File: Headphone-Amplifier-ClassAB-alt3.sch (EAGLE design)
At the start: 17 parts, among them T1 2N3904, T2 2N3904, T3 2N3906

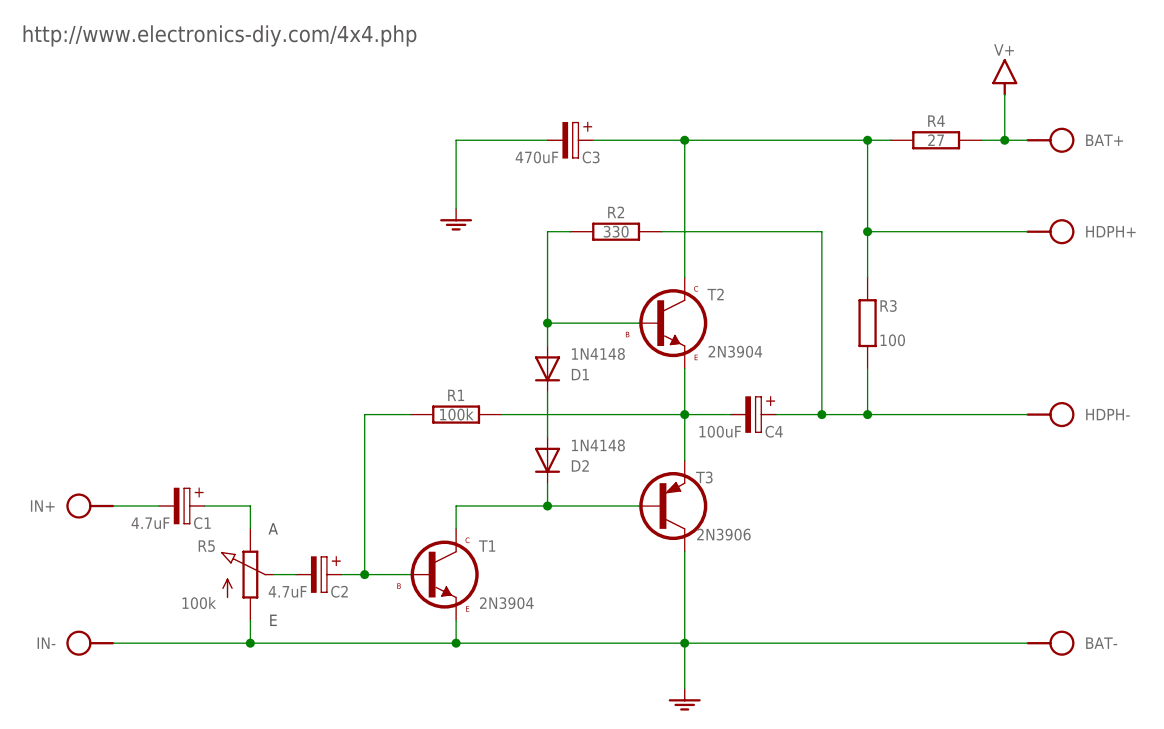
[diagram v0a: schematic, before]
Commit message: ...
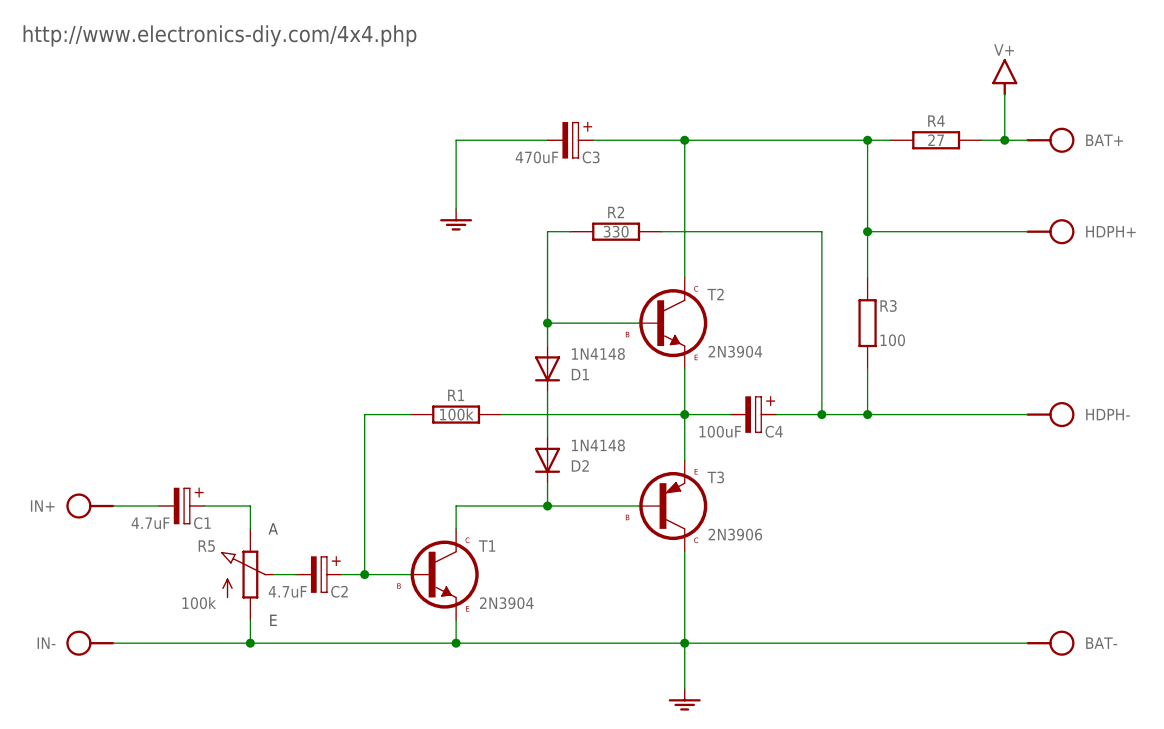
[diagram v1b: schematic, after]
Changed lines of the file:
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@@
     <grid distance="0.1" unitdist="inch" unit="inch" style="lines" multiple="1" display="yes" altdistance="2" altunitdist="inch" altunit="inch" />
     <layers>
-      <layer number="1" name="Top" color="4" fill="1" visible="yes" active="no" />
-      <layer number="2" name="Route2" color="1" fill="3" visible="yes" active="no" />
-      <layer number="3" name="Route3" color="4" fill="3" visible="yes" active="no" />
-      <layer number="4" name="Route4" color="1" fill="4" visible="yes" active="no" />
-      <layer number="5" name="Route5" color="4" fill="4" visible="yes" active="no" />
-      <layer number="6" name="Route6" color="1" fill="8" visible="yes" active="no" />
-      <layer number="7" name="Route7" color="4" fill="8" visible="yes" active="no" />
-      <layer number="8" name="Route8" color="1" fill="2" visible="yes" active="no" />
-      <layer number="9" name="Route9" color="4" fill="2" visible="yes" active="no" />
-      <layer number="10" name="Route10" color="1" fill="7" visible="yes" active="no" />
-      <layer number="11" name="Route11" color="4" fill="7" visible="yes" active="no" />
-      <layer number="12" name="Route12" color="1" fill="5" visible="yes" active="no" />
-      <layer number="13" name="Route13" color="4" fill="5" visible="yes" active="no" />
-      <layer number="14" name="Route14" color="1" fill="6" visible="yes" active="no" />
-      <layer number="15" name="Route15" color="4" fill="6" visible="yes" active="no" />
-      <layer number="16" name="Bottom" color="1" fill="1" visible="yes" active="no" />
-      <layer number="17" name="Pads" color="2" fill="1" visible="yes" active="no" />
-      <layer number="18" name="Vias" color="2" fill="1" visible="yes" active="no" />
-      <layer number="19" name="Unrouted" color="6" fill="1" visible="yes" active="no" />
-      <layer number="20" name="Dimension" color="24" fill="1" visible="yes" active="no" />
-      <layer number="21" name="tPlace" color="16" fill="1" visible="yes" active="no" />
-      <layer number="22" name="bPlace" color="14" fill="1" visible="yes" active="no" />
-      <layer number="23" name="tOrigins" color="15" fill="1" visible="yes" active="no" />
-      <layer number="24" name="bOrigins" color="15" fill="1" visible="yes" active="no" />
-      <layer number="25" name="tNames" color="7" fill="1" visible="yes" active="no" />
-      <layer number="26" name="bNames" color="7" fill="1" visible="yes" active="no" />
-      <layer number="27" name="tValues" color="7" fill="1" visible="yes" active="no" />
-      <layer number="28" name="bValues" color="7" fill="1" visible="yes" active="no" />
+      <layer number="1" name="Top" color="4" fill="1" visible="no" active="no" />
+      <layer number="2" name="Route2" color="1" fill="3" visible="no" active="no" />
+      <layer number="3" name="Route3" color="4" fill="3" visible="no" active="no" />
+      <layer number="4" name="Route4" color="1" fill="4" visible="no" active="no" />
+      <layer number="5" name="Route5" color="4" fill="4" visible="no" active="no" />
+      <layer number="6" name="Route6" color="1" fill="8" visible="no" active="no" />
+      <layer number="7" name="Route7" color="4" fill="8" visible="no" active="no" />
+      <layer number="8" name="Route8" color="1" fill="2" visible="no" active="no" />
+      <layer number="9" name="Route9" color="4" fill="2" visible="no" active="no" />
+      <layer number="10" name="Route10" color="1" fill="7" visible="no" active="no" />
+      <layer number="11" name="Route11" color="4" fill="7" visible="no" active="no" />
+      <layer number="12" name="Route12" color="1" fill="5" visible="no" active="no" />
+      <layer number="13" name="Route13" color="4" fill="5" visible="no" active="no" />
+      <layer number="14" name="Route14" color="1" fill="6" visible="no" active="no" />
+      <layer number="15" name="Route15" color="4" fill="6" visible="no" active="no" />
+      <layer number="16" name="Bottom" color="1" fill="1" visible="no" active="no" />
+      <layer number="17" name="Pads" color="2" fill="1" visible="no" active="no" />
+      <layer number="18" name="Vias" color="2" fill="1" visible="no" active="no" />
+      <layer number="19" name="Unrouted" color="6" fill="1" visible="no" active="no" />
+      <layer number="20" name="Dimension" color="24" fill="1" visible="no" active="no" />
+      <layer number="21" name="tPlace" color="16" fill="1" visible="no" active="no" />
+      <layer number="22" name="bPlace" color="14" fill="1" visible="no" active="no" />
+      <layer number="23" name="tOrigins" color="15" fill="1" visible="no" active="no" />
+      <layer number="24" name="bOrigins" color="15" fill="1" visible="no" active="no" />
+      <layer number="25" name="tNames" color="7" fill="1" visible="no" active="no" />
+      <layer number="26" name="bNames" color="7" fill="1" visible="no" active="no" />
+      <layer number="27" name="tValues" color="7" fill="1" visible="no" active="no" />
+      <layer number="28" name="bValues" color="7" fill="1" visible="no" active="no" />
       <layer number="29" name="tStop" color="7" fill="3" visible="no" active="no" />
       <layer number="30" name="bStop" color="7" fill="6" visible="no" active="no" />
@@
       <layer number="35" name="tGlue" color="7" fill="4" visible="no" active="no" />
       <layer number="36" name="bGlue" color="7" fill="5" visible="no" active="no" />
-      <layer number="37" name="tTest" color="7" fill="1" visible="yes" active="no" />
-      <layer number="38" name="bTest" color="7" fill="1" visible="yes" active="no" />
+      <layer number="37" name="tTest" color="7" fill="1" visible="no" active="no" />
+      <layer number="38" name="bTest" color="7" fill="1" visible="no" active="no" />
       <layer number="39" name="tKeepout" color="4" fill="11" visible="no" active="no" />
       <layer number="40" name="bKeepout" color="1" fill="11" visible="no" active="no" />
@@
       <layer number="44" name="Drills" color="7" fill="1" visible="no" active="no" />
       <layer number="45" name="Holes" color="7" fill="1" visible="no" active="no" />
-      <layer number="46" name="Milling" color="3" fill="1" visible="yes" active="no" />
-      <layer number="47" name="Measures" color="7" fill="1" visible="yes" active="no" />
-      <layer number="48" name="Document" color="7" fill="1" visible="yes" active="no" />
-      <layer number="49" name="Reference" color="7" fill="1" visible="yes" active="no" />
-      <layer number="51" name="tDocu" color="6" fill="1" visible="yes" active="no" />
-      <layer number="52" name="bDocu" color="7" fill="1" visible="yes" active="no" />
+      <layer number="46" name="Milling" color="3" fill="1" visible="no" active="no" />
+      <layer number="47" name="Measures" color="7" fill="1" visible="no" active="no" />
+      <layer number="48" name="Document" color="7" fill="1" visible="no" active="no" />
+      <layer number="49" name="Reference" color="7" fill="1" visible="no" active="no" />
+      <layer number="51" name="tDocu" color="6" fill="1" visible="no" active="no" />
+      <layer number="52" name="bDocu" color="7" fill="1" visible="no" active="no" />
       <layer number="90" name="Modules" color="5" fill="1" visible="yes" active="yes" />
       <layer number="91" name="Nets" color="2" fill="1" visible="yes" active="yes" />
